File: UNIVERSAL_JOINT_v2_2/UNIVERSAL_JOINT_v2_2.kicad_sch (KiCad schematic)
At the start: 127 parts, among them J1 Conn_02x07_Odd_Even, J10 n.m., J9 HEADER_MALE_2X3_2.54_SMT, Q1 IAUC120N06S5L, Q2 IAUC120N06S5L, Q3 IAUC120N06S5L, Q4 IAUC120N06S5L, Q5 IAUC120N06S5L, Q6 IAUC120N06S5L, Q7 ZXTP19100CFFCT, Q8 IAUC120N06S5L, SW1 SKHMPE010, T1 2PC4081S,115, T2 2PC4081S,115, U1 DRV8323RHRGZR, U2 TCAN332G, U3 STM32G431C8T6, U4 MA730, X1 LFXTAL069392CUTT

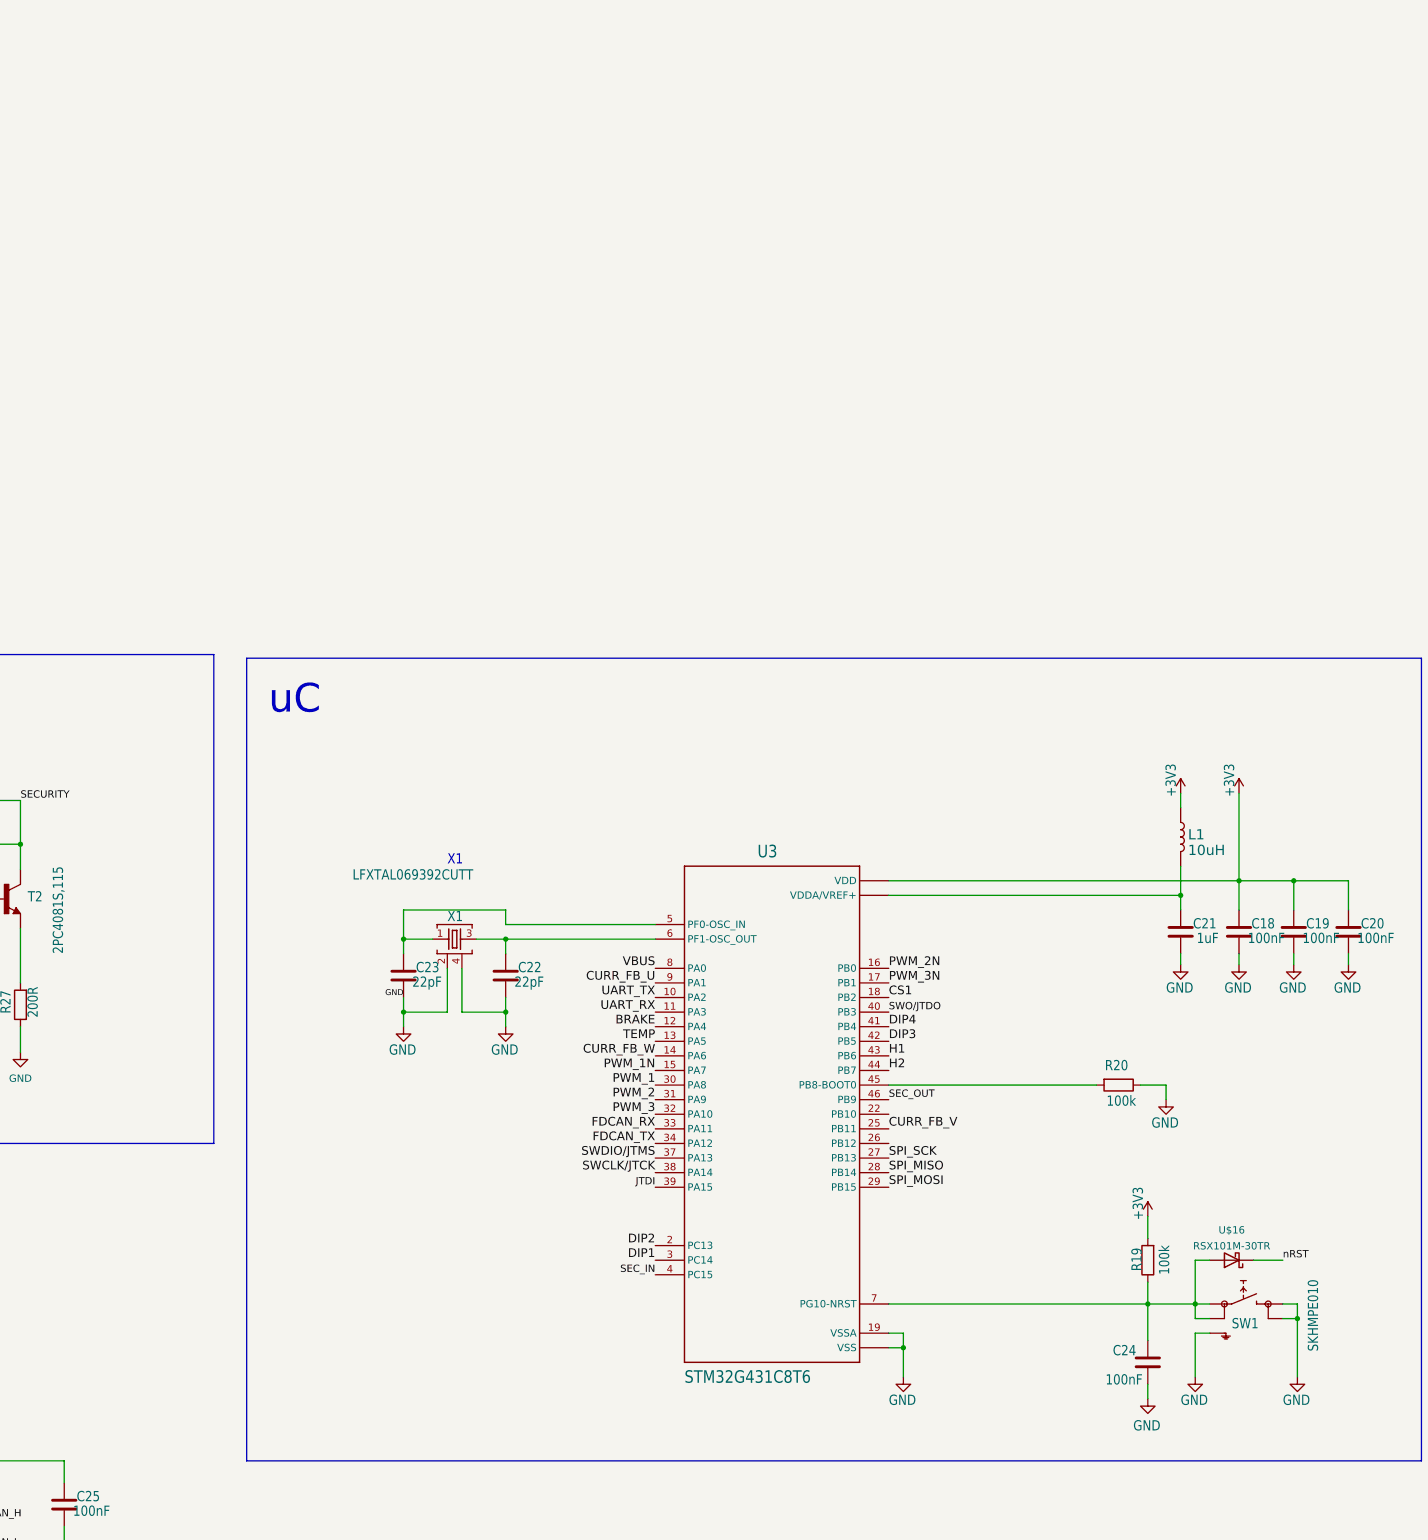
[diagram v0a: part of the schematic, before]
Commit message: udpate
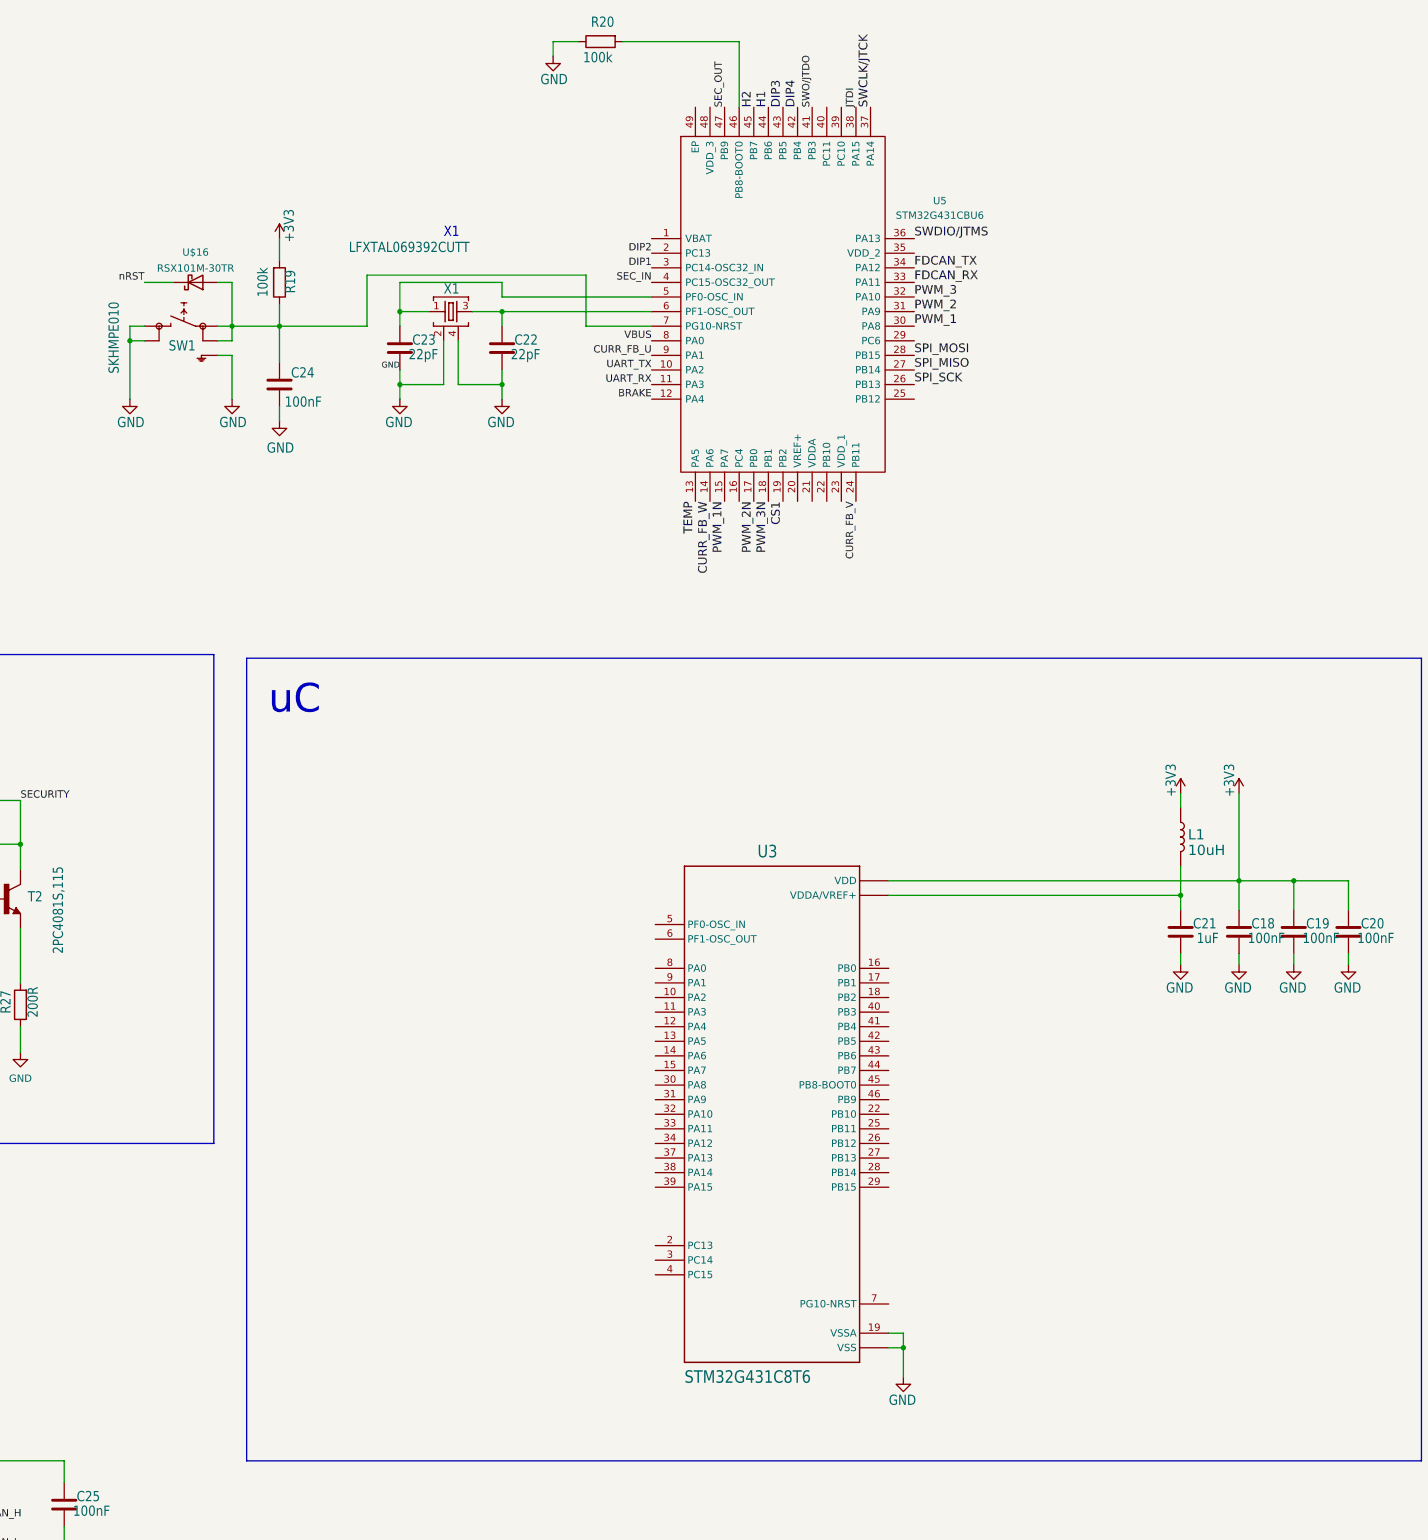
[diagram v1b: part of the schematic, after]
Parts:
- added U5: STM32G431CBU6, UNIVERSAL_JOINT:QFN50P700X700X65-49N-D, symbol STM32G431CBU6:STM32G431CBU6
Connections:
- net BRAKE: now also U5.12 (PA4); no longer U3.12 (PA4)
- net CS1: now also U5.19 (PB2); no longer U3.18 (PB2)
- net CURR_FB_U: now also U5.9 (PA1); no longer U3.9 (PA1)
- net CURR_FB_V: now also U5.24 (PB11); no longer U3.25 (PB11)
- net CURR_FB_W: now also U5.14 (PA6); no longer U3.14 (PA6)
- net DIP1: now also U5.3 (PC14-OSC32_IN); no longer U3.3 (PC14)
- net DIP2: now also U5.2 (PC13); no longer U3.2 (PC13)
- net DIP3: now also U5.43 (PB5); no longer U3.42 (PB5)
- net DIP4: now also U5.42 (PB4); no longer U3.41 (PB4)
- net FDCAN_RX: now also U5.33 (PA11); no longer U3.33 (PA11)
- net FDCAN_TX: now also U5.34 (PA12); no longer U3.34 (PA12)
- net H1: now also U5.44 (PB6); no longer U3.43 (PB6)
- net H2: now also U5.45 (PB7); no longer U3.44 (PB7)
- net JTDI: now also U5.38 (PA15); no longer U3.39 (PA15)
- net PWM_1: now also U5.30 (PA8); no longer U3.30 (PA8)
- net PWM_1N: now also U5.15 (PA7); no longer U3.15 (PA7)
- net PWM_2: now also U5.31 (PA9); no longer U3.31 (PA9)
- net PWM_2N: now also U5.17 (PB0); no longer U3.16 (PB0)
- net PWM_3: now also U5.32 (PA10); no longer U3.32 (PA10)
- net PWM_3N: now also U5.18 (PB1); no longer U3.17 (PB1)
- net SEC_IN: now also U5.4 (PC15-OSC32_OUT); no longer U3.4 (PC15)
- net SEC_OUT: now also U5.47 (PB9); no longer U3.46 (PB9)
- net SPI_MISO: now also U5.27 (PB14); no longer U3.28 (PB14)
- net SPI_MOSI: now also U5.28 (PB15); no longer U3.29 (PB15)
- net SPI_SCK: now also U5.26 (PB13); no longer U3.27 (PB13)
- net SWCLK/JTCK: now also U5.37 (PA14); no longer U3.38 (PA14)
- net SWDIO/JTMS: now also U5.36 (PA13); no longer U3.37 (PA13)
- net SWO/JTDO: now also U5.41 (PB3); no longer U3.40 (PB3)
- net TEMP: now also U5.13 (PA5); no longer U3.13 (PA5)
- net UART_RX: now also U5.11 (PA3); no longer U3.11 (PA3)
- net UART_TX: now also U5.10 (PA2); no longer U3.10 (PA2)
- net VBUS: now also U5.8 (PA0); no longer U3.8 (PA0)
- net at C23.2, X1.1: now also U5.5 (PF0-OSC_IN); no longer U3.5 (PF0-OSC_IN)
- net at C22.2, X1.3: now also U5.6 (PF1-OSC_OUT); no longer U3.6 (PF1-OSC_OUT)
- net at R20.2: now also U5.46 (PB8-BOOT0); no longer U3.45 (PB8-BOOT0)
- net at C24.2, R19.1, SW1.1 (1.1)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: now also U5.7 (PG10-NRST); no longer U3.7 (PG10-NRST)
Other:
- moved on the sheet: C22, C23, C24, R19, R20, SW1, U$16, X1
